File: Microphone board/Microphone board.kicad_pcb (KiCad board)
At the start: 4 copper layers, 155 parts, among them J1 TF-01A, J2 OV2640, J3 NHD-2.4-240320AF-CSXP, J4 TYPE-C 16PIN 2MD(073), M1 MSM261DDB019, M10 MSM261DDB019, M11 MSM261DDB019, M12 MSM261DDB019, M13 MSM261DDB019, M14 MSM261DDB019, M15 MSM261DDB019, M16 MSM261DDB019, M2 MSM261DDB019, M3 MSM261DDB019, M4 MSM261DDB019, M5 MSM261DDB019, M6 MSM261DDB019, M7 MSM261DDB019, M8 MSM261DDB019, M9 MSM261DDB019, Q1 AO3401A, Q2 MMBT3904, U1 STM32H747XIH6, U2 24LC256, U3 TLV320ADC5140IRTWT, U4 TLV320ADC5140IRTWT, U5 TPD6F003, U6 USBLC6-2SC6, U7 AP63203WU, U8 TPS7A2033PDBV, U9 TPS2116DRL, Y1 SX2M25.000M20F30TNN

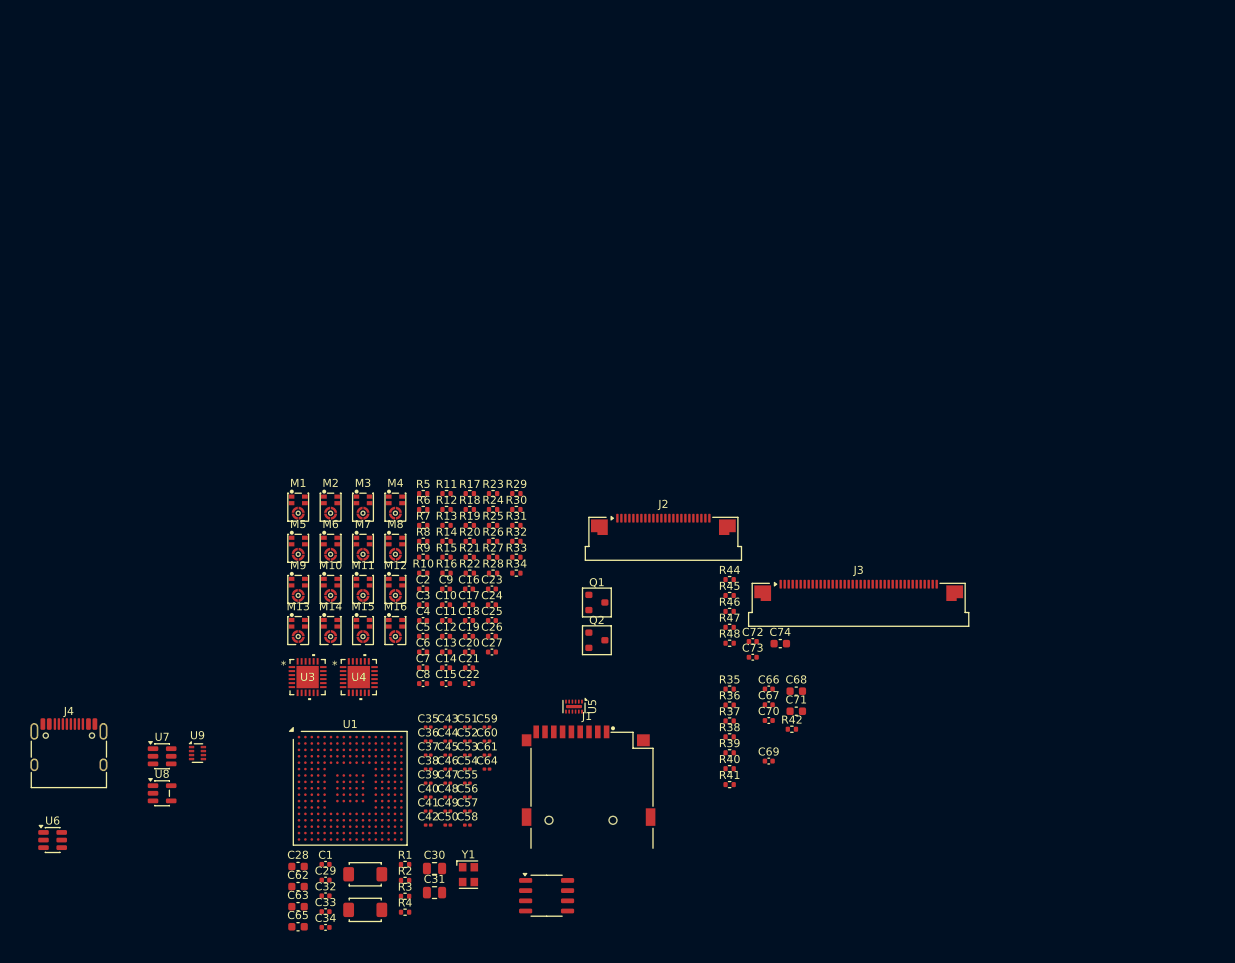
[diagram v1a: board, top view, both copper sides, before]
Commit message: PCB routed
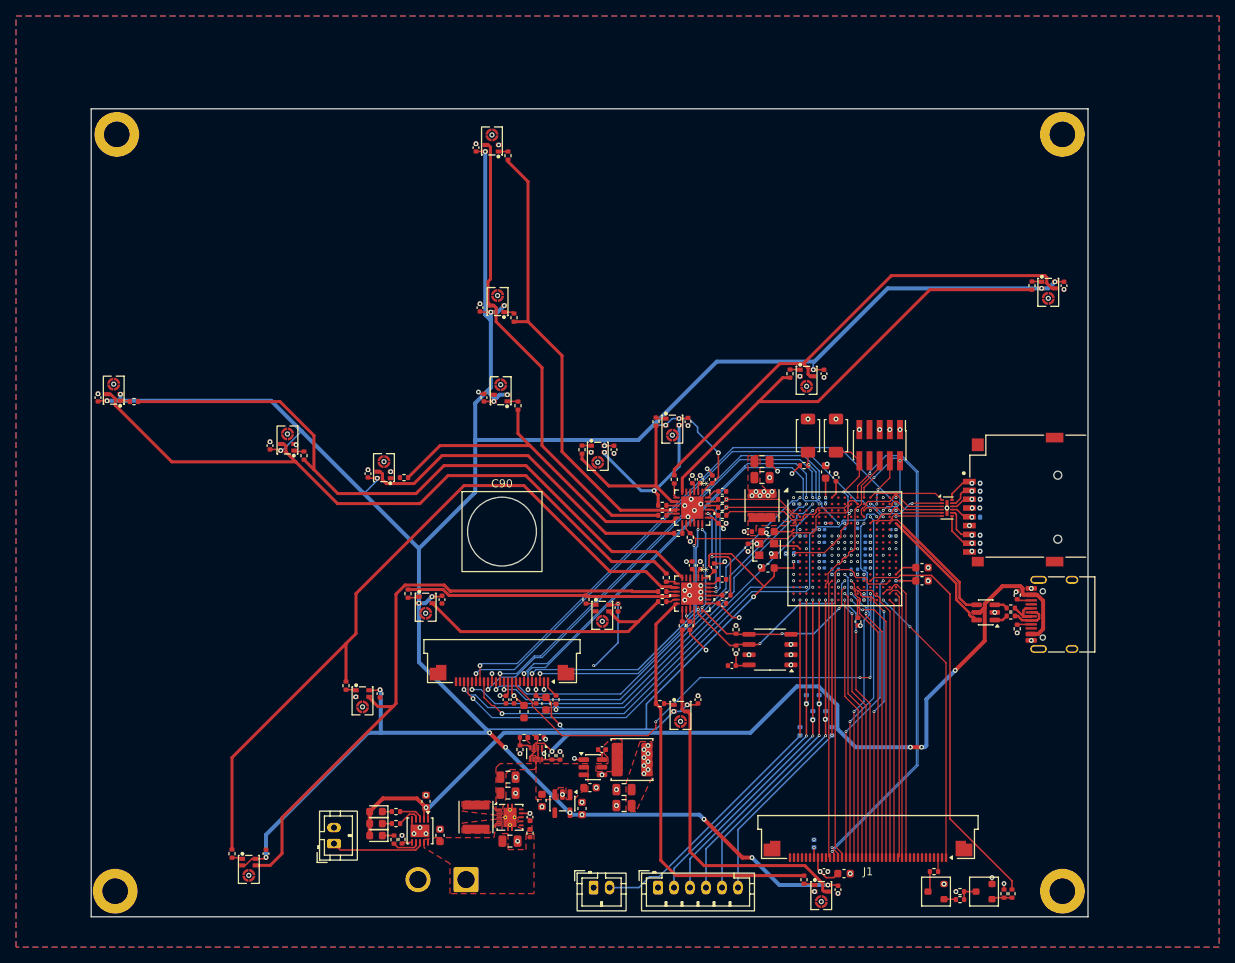
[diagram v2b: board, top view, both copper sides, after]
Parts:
- added BT1: 3.7V 18650, Connector_Wire:SolderWire-1.5sqmm_1x02_P6mm_D1.7mm_OD3mm, F.Cu at (106.2, 135.8)
- added C75: 10u 6.3V, Capacitor_SMD:C_0805_2012Metric, F.Cu at (111.7, 130.9)
- added C76: 100n, Capacitor_SMD:C_0402_1005Metric, F.Cu at (114.2, 127.9)
- added C77: 2.2u, Capacitor_SMD:C_0402_1005Metric, F.Cu at (115.5, 118.0)
- added C78: 10u 6.3V, Capacitor_SMD:C_0805_2012Metric, F.Cu at (111.5, 122.9)
- added C79: 10u 6.3V, Capacitor_SMD:C_0805_2012Metric, F.Cu at (111.5, 124.9)
- added C80: 10u, Capacitor_SMD:C_0603_1608Metric, F.Cu at (121.8, 124.2)
- added C81: 100n, Capacitor_SMD:C_0402_1005Metric, F.Cu at (123.2, 119.5)
- added C82: 22u, Capacitor_SMD:C_0805_2012Metric, F.Cu at (126.0, 124.5)
- added C83: 22u, Capacitor_SMD:C_0805_2012Metric, F.Cu at (126.0, 126.5)
- added C84: 2.2u, Capacitor_SMD:C_0603_1608Metric, F.Cu at (115.8, 125.9)
- added C85: 2.2u, Capacitor_SMD:C_0603_1608Metric, F.Cu at (120.8, 126.9)
- added C86: 1u, Capacitor_SMD:C_0603_1608Metric, F.Cu at (101.2, 126.0)
- added C87: 1u, Capacitor_SMD:C_0603_1608Metric, F.Cu at (103.0, 130.2)
- added C88: 100n, Capacitor_SMD:C_0402_1005Metric, B.Cu at (170.0, 89.3)
- added C89: 100n, Capacitor_SMD:C_0201_0603Metric, B.Cu at (160.3, 98.4)
- added C90: OV2640, Mic_Parts:OV2640, F.Cu at (110.8, 92.2)
- added D1: Green, PCM_JLCPCB:D_0603, F.Cu at (95.0, 130.2)
- added D2: Yellow, PCM_JLCPCB:D_0603, F.Cu at (95.0, 128.8)
- added D3: Red, PCM_JLCPCB:D_0603, F.Cu at (95.0, 127.2)
- added H1: M3 mounting hole, MountingHole:MountingHole_3.2mm_M3_DIN965_Pad, F.Cu at (62.6, 42.6)
- added H2: M3 mounting hole, MountingHole:MountingHole_3.2mm_M3_DIN965_Pad, F.Cu at (62.4, 137.2)
- added H3: M3 mounting hole, MountingHole:MountingHole_3.2mm_M3_DIN965_Pad, F.Cu at (180.8, 137.2)
- added H4: M3 mounting hole, MountingHole:MountingHole_3.2mm_M3_DIN965_Pad, F.Cu at (180.8, 42.6)
- added J5: Trigger, Connector_JST:JST_PH_B2B-PH-K_1x02_P2.00mm_Vertical, F.Cu at (122.2, 136.8)
- added J6: Menu, Connector_JST:JST_PH_B6B-PH-K_1x06_P2.00mm_Vertical, F.Cu at (130.2, 136.8)
- added J7: Conn_ARM_JTAG_SWD_10, Connector_PinHeader_1.27mm:PinHeader_2x05_P1.27mm_Vertical_SMD, F.Cu at (158.0, 81.5)
- added L1: GNR4018S2R2MT, Inductor_SMD:L_Abracon_ASPI-4030S, F.Cu at (143.2, 89.0)
- added L2: GNR4018S2R2MT, Inductor_SMD:L_Abracon_ASPI-4030S, F.Cu at (107.5, 127.9)
- added L3: FNR5040S4R7MT, Inductor_SMD:L_Changjiang_FNR5040S, F.Cu at (127.0, 120.8)
- added R43: 10k, Resistor_SMD:R_0402_1005Metric, B.Cu at (170.0, 90.5)
- added R49: 100k, Resistor_SMD:R_0402_1005Metric, F.Cu at (113.0, 119.5)
- added R50: 100R, Resistor_SMD:R_0402_1005Metric, F.Cu at (114.2, 129.9)
- added R51: 10k, Resistor_SMD:R_0402_1005Metric, F.Cu at (117.0, 120.2)
- added R52: 15k, Resistor_SMD:R_0402_1005Metric, F.Cu at (118.0, 120.2)
- added R53: 470R, Resistor_SMD:R_0402_1005Metric, F.Cu at (97.5, 127.2)
- added R54: 470R, Resistor_SMD:R_0402_1005Metric, F.Cu at (97.5, 128.8)
- added R55: 470R, Resistor_SMD:R_0402_1005Metric, F.Cu at (97.2, 130.8)
- added R56: 5k1, Resistor_SMD:R_0402_1005Metric, F.Cu at (175.2, 104.4)
- added R57: 5k1, Resistor_SMD:R_0402_1005Metric, F.Cu at (175.2, 100.2)
- added R58: 22R, Resistor_SMD:R_0402_1005Metric, F.Cu at (174.3, 102.8)
- added R59: 22R, Resistor_SMD:R_0402_1005Metric, F.Cu at (174.3, 101.8)
- added R60: 1k, Resistor_SMD:R_0402_1005Metric, F.Cu at (98.2, 130.7)
- added R61: 10k, Resistor_SMD:R_0402_1005Metric, B.Cu at (148.0, 117.2)
- added R62: 10k, Resistor_SMD:R_0402_1005Metric, B.Cu at (152.0, 117.2)
- added R63: 10k, Resistor_SMD:R_0402_1005Metric, B.Cu at (151.2, 115.2)
- added R64: 10k, Resistor_SMD:R_0402_1005Metric, B.Cu at (150.4, 113.2)
- added R65: 10k, Resistor_SMD:R_0402_1005Metric, B.Cu at (149.6, 115.2)
- added R66: 10k, Resistor_SMD:R_0402_1005Metric, B.Cu at (148.8, 113.2)
- added TH1: 10k, Connector_JST:JST_PH_B2B-PH-K_1x02_P2.00mm_Vertical, F.Cu at (89.8, 131.2)
- added U10: TPS7A2033PDBV, Package_TO_SOT_SMD:SOT-23-5, F.Cu at (118.3, 126.2)
- added U11: USBLC6-2SC6, Package_TO_SOT_SMD:SOT-23-6, F.Cu at (171.2, 102.3)
- C1: value 100n -> 220pF
- C10, C11, C12, C13, C14, C16, C17, C18, C19, C20, C21, C22, C23, C24, C25, C26, C27, C8, C9: footprint Capacitor_SMD:C_0402_1005Metric -> Capacitor_SMD:C_0201_0603Metric; moved to B.Cu
- C15: value 100n -> 1u; footprint Capacitor_SMD:C_0402_1005Metric -> Capacitor_SMD:C_0603_1608Metric
- C2: footprint Capacitor_SMD:C_0402_1005Metric -> Capacitor_SMD:C_0603_1608Metric
- C28: value 4.7u -> 100n; footprint Capacitor_SMD:C_0603_1608Metric -> Capacitor_SMD:C_0201_0603Metric; moved to B.Cu
- C29: value 220pF -> 100n; footprint Capacitor_SMD:C_0402_1005Metric -> Capacitor_SMD:C_0201_0603Metric; moved to B.Cu
- C30, C31: value 10u -> 100n; footprint Capacitor_SMD:C_0805_2012Metric -> Capacitor_SMD:C_0201_0603Metric; moved to B.Cu
- C32, C33, C34: value 2.2u -> 100n; footprint Capacitor_SMD:C_0402_1005Metric -> Capacitor_SMD:C_0201_0603Metric; moved to B.Cu
- C35, C36, R1, R41, R42: moved to B.Cu
- C37: value 100n -> 4.7u; footprint Capacitor_SMD:C_0201_0603Metric -> Capacitor_SMD:C_0603_1608Metric
- C38: value 100n -> 1u; footprint Capacitor_SMD:C_0201_0603Metric -> Capacitor_SMD:C_0603_1608Metric
- C39, C40, C41, C42, C43, C44, C45, C46, C47, C48, C49, C50, C51, C52, C53, C54, C55, C56, C59, C60, C64: footprint Capacitor_SMD:C_0201_0603Metric -> Capacitor_SMD:C_0402_1005Metric
- C4, C69: value 100n -> 4.7u; footprint Capacitor_SMD:C_0402_1005Metric -> Capacitor_SMD:C_0603_1608Metric
- C57, C58, C61: value 100n -> 2.2u; footprint Capacitor_SMD:C_0201_0603Metric -> Capacitor_SMD:C_0402_1005Metric
- C6: value 100n -> 10u; footprint Capacitor_SMD:C_0402_1005Metric -> Capacitor_SMD:C_0805_2012Metric
- C62: value 4.7u -> 2.2u; footprint Capacitor_SMD:C_0603_1608Metric -> Capacitor_SMD:C_0402_1005Metric
- C63, C65: value 1u -> 100n; footprint Capacitor_SMD:C_0603_1608Metric -> Capacitor_SMD:C_0402_1005Metric
- C68: value 4.7u -> 100n; footprint Capacitor_SMD:C_0603_1608Metric -> Capacitor_SMD:C_0402_1005Metric; moved to B.Cu
- C7: value 2.2u -> 10u; footprint Capacitor_SMD:C_0402_1005Metric -> Capacitor_SMD:C_0805_2012Metric
- J1: value TF-01A -> NHD-2.4-240320AF-CSXP; footprint Mic_Parts:TF-01A -> Connector_FFC-FPC:Amphenol_F32R-1A7x1-11040_1x40-1MP_P0.5mm_Horizontal
- J2: footprint Connector_FFC-FPC:Amphenol_F32R-1A7x1-11024_1x24-1MP_P0.5mm_Horizontal -> Connector_FFC-FPC:Amphenol_F32Q-1A7x1-11024_1x24-1MP_P0.5mm_Horizontal
- J3: value NHD-2.4-240320AF-CSXP -> TF-01A; footprint Connector_FFC-FPC:Amphenol_F32R-1A7x1-11040_1x40-1MP_P0.5mm_Horizontal -> Mic_Parts:TF-01A
- Q1: value AO3401A -> MMBT3904
- Q2: value MMBT3904 -> AO3401A
- R10, R11, R12, R13, R14, R15, R16, R17, R18, R19, R20, R21, R22, R23, R24, R29, R30, R31, R32, R7, R8, R9: value 33R -> 22R
- R2: value 10k -> 2k2
- R33, R34: value 33R -> 10k
- R35: value 10k -> 1k
- R37: value 10k -> 4k7
- R38: value 10k -> 10R
- R39: value 10k -> 2R
- R4: value 2k2 -> 10k
- R44: value 10R -> 10k; moved to B.Cu
- R45: value 4k7 -> 10k; moved to B.Cu
- R46: value 2R -> 10k; moved to B.Cu
- R47: value 1k -> 10k; moved to B.Cu
- R48: value 10k -> 240k
- R5, R6: value 10k -> 22R
- U6: value USBLC6-2SC6 -> TPS63001; footprint Package_TO_SOT_SMD:SOT-23-6 -> Package_SON:Texas_DRC0010J_ThermalVias
- U7: value AP63203WU -> TPS2116DRL; footprint Package_TO_SOT_SMD:TSOT-23-6 -> Package_TO_SOT_SMD:SOT-583-8
- U8: value TPS7A2033PDBV -> AP63203WU; footprint Package_TO_SOT_SMD:SOT-23-5 -> Package_TO_SOT_SMD:TSOT-23-6
- U9: value TPS2116DRL -> MCP73833-xxx-MF; footprint Package_TO_SOT_SMD:SOT-583-8 -> Package_DFN_QFN:DFN-10-1EP_3x3mm_P0.5mm_EP1.58x2.35mm
- moved J4 125.6 mm to (180.9, 102.6), turned to 90 degrees
- moved C49 101.2 mm to (181.0, 61.5), turned to -90 degrees
- moved M1 97.5 mm to (179.0, 63.1)
- moved C32 84.0 mm to (159.7, 92.8), turned to 180 degrees
- moved C28 82.3 mm to (156.5, 92.8), turned to 180 degrees
- moved C34 82.2 mm to (151.2, 88.3), turned to -90 degrees
- moved S2 81.1 mm to (149.0, 80.2), turned to -90 degrees
- moved S1 80.4 mm to (152.5, 80.2), turned to 90 degrees
- moved C29 79.4 mm to (156.5, 94.4), turned to 180 degrees
- moved R13 79.1 mm to (177.0, 61.5), turned to -90 degrees
- moved C33 77.3 mm to (150.7, 93.6)
- moved C65 76.2 mm to (137.0, 85.7), turned to 90 degrees
- moved R4 74.9 mm to (148.5, 84.0), turned to 180 degrees
- moved C41 73.7 mm to (151.0, 72.5), turned to -90 degrees
- moved C31 73.1 mm to (159.7, 92.0), turned to 180 degrees
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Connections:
- net Net-(J4-D+-PadA6) renamed /USB/USB_IN_P
- net Net-(J4-D--PadA7) renamed /USB/USB_IN_N
- C1 pad 1: +3V3 -> Net-(U1A-VLXSMPS)
- C10 pad 1: +3V3A -> +3V3
- C12 pad 1: +3V3A -> +3V3
- C13 pad 1: +3V3A -> +3V3
- C14 pad 1: +3V3A -> +3V3
- C16 pad 1: +3V3A -> +3V3
- C17 pad 1: +3V3A -> +3V3
- C18 pad 1: +3V3A -> +3V3
- C19 pad 1: +3V3A -> +3V3
- C2 pad 1: Net-(U3B-AREG) -> Net-(U1A-VCAPDSI)
- C20 pad 1: +3V3A -> +3V3
- C21 pad 1: +3V3A -> +3V3
- C22 pad 1: +3V3A -> +3V3
- C23 pad 1: +3V3A -> +3V3
- C24 pad 1: +3V3A -> +3V3
- C27 pad 1: +3V3A -> +3V3
- C28 pad 1: Net-(U1A-VDDSMPS) -> +3V3
- C29 pad 1: Net-(U1A-VLXSMPS) -> +3V3
- C3 pad 1: Net-(U4B-AREG) -> Net-(C3-Pad1)
- C32 pad 1: Net-(C32-Pad1) -> +3V3
- C33 pad 1: Net-(C32-Pad1) -> +3V3
- C34 pad 1: Net-(U1A-VCAPDSI) -> +3V3
- C4 pad 1: Net-(U3B-VREF) -> Net-(U1A-VDDSMPS)
- C41 pad 1: +3V3 -> +3V3A
- C42 pad 1: +3V3 -> +3V3A
- C43 pad 1: +3V3 -> +3V3A
- C44 pad 1: +3V3 -> +3V3A
- C45 pad 1: +3V3 -> +3V3A
- C46 pad 1: +3V3 -> +3V3A
- C47 pad 1: +3V3 -> +3V3A
- C48 pad 1: +3V3 -> +3V3A
- C49 pad 1: +3V3 -> +3V3A
- C5 pad 1: Net-(U3B-DREG) -> Net-(C3-Pad1)
- C50 pad 1: +3V3 -> +3V3A
- C51 pad 1: +3V3 -> +3V3A
- C52 pad 1: +3V3 -> +3V3A
- C53 pad 1: +3V3 -> +3V3A
- C54 pad 1: +3V3 -> +3V3A
- C55 pad 1: +3V3 -> +3V3A
- C56 pad 1: +3V3 -> +3V3A
- C57 pad 1: +3V3 -> Net-(U3B-AREG)
- C58 pad 1: +3V3 -> Net-(U4B-AREG)
- C59 pad 1: +3V3 -> Net-(U3B-VREF)
- C6 pad 1: Net-(U4B-VREF) -> +3V3
- C60 pad 1: +3V3 -> Net-(U4B-VREF)
- C61 pad 1: +3V3 -> Net-(U3B-DREG)
- C62 pad 1: +3V3 -> Net-(U4B-DREG)
- C64 pad 1: +3V3A -> +3V3
- C66 pad 1: +3V3 -> +3V3A
- C7 pad 1: Net-(U4B-DREG) -> +3V3
- C8 pad 1: +3V3A -> +3V3
- C9 pad 1: +3V3A -> +3V3
- J1 pad 1: Net-(J1-DAT2) -> /MCU/TEAR
- J1 pad 2: Net-(J1-DAT3/CD) -> GND
- J1 pad 3: Net-(J1-CMD) -> /Display/LIGHT
- J1 pad 4: +3V3 -> GND
- J1 pad 5: Net-(J1-CLK) -> GND
- J1 pad 7: Net-(J1-DAT0) -> GND
- J1 pad 8: Net-(J1-DAT1) -> GND
- J1 pad 9: /MCU/SD_DET -> GND
- J2 pad 18: /MCU/DCMI_D7 -> /MCU/DCMI_D4
- J3 pad 1: GND -> /SD/SD_D2F
- J3 pad 2: unconnected-(J3-Pin_2-Pad2) -> /SD/SD_D3F
- J3 pad 3: unconnected-(J3-Pin_3-Pad3) -> /SD/SD_CMDF
- J3 pad 4: unconnected-(J3-Pin_4-Pad4) -> +3V3
- J3 pad 5: unconnected-(J3-Pin_5-Pad5) -> /SD/SD_CLKF
- J3 pad 6: unconnected-(J3-Pin_6-Pad6) -> GND
- J3 pad 7: +3V3 -> /SD/SD_D0F
- J3 pad 8: +3V3 -> /SD/SD_D1F
- J3 pad 9: GND -> /MCU/SD_DET
- M10 pad 4: /Microphones/CH6_CLK -> /Microphones/CH5_CLK
- M11 pad 2: GND -> +3V3A
- M11 pad 4: /Microphones/CH7_CLK -> /Microphones/CH6_CLK
- M12 pad 4: /Microphones/CH8_CLK -> /Microphones/CH6_CLK
- M13 pad 4: unconnected-(M13-CLK-Pad4) -> /Microphones/CH7_CLK
- M14 pad 2: +3V3A -> GND
- M14 pad 4: /Microphones/CH5_CLK -> /Microphones/CH7_CLK
- M15 pad 4: /Microphones/CH6_CLK -> /Microphones/CH8_CLK
- M16 pad 2: +3V3A -> GND
- M3 pad 2: GND -> +3V3A
- M4 pad 2: +3V3A -> GND
- M5 pad 2: GND -> +3V3A
- M6 pad 4: /Microphones/CH4_CLK -> /Microphones/CH3_CLK
- M7 pad 4: /Microphones/CH3_CLK -> /Microphones/CH4_CLK
- M8 pad 2: +3V3A -> GND
- M9 pad 2: GND -> +3V3A
- Q1 pad 1: Net-(Q1-G) -> Net-(Q1-B)
- Q1 pad 2: +3V3 -> GND
- Q1 pad 3: Net-(Q1-D) -> Net-(Q1-C)
- Q2 pad 1: Net-(Q2-B) -> Net-(Q2-G)
- Q2 pad 2: GND -> +3V3
- Q2 pad 3: Net-(Q2-C) -> Net-(Q2-D)
- R1 pad 1: /MCU/BOOT0 -> +3V3
- R1 pad 2: GND -> /MCU/NRST
- R10 pad 1: /Microphones/CH4_CLK -> Net-(M12-DAT)
- R10 pad 2: Net-(U3A-IN4M_GPO4) -> /Microphones/CH6_DAT
- R11 pad 1: /Microphones/CH5_CLK -> Net-(M14-DAT)
- R11 pad 2: Net-(U4A-IN1M_GPO1) -> /Microphones/CH7_DAT
- R12 pad 1: /Microphones/CH6_CLK -> Net-(M16-DAT)
- R12 pad 2: Net-(U4A-IN2M_GPO2) -> /Microphones/CH8_DAT
- R13 pad 1: /Microphones/CH7_CLK -> Net-(M1-DAT)
- R13 pad 2: Net-(U4A-IN3M_GPO3) -> /Microphones/CH1_DAT
- R14 pad 1: /Microphones/CH8_CLK -> Net-(M3-DAT)
- R14 pad 2: Net-(U4A-IN4M_GPO4) -> /Microphones/CH2_DAT
- R15 pad 1: Net-(M1-DAT) -> Net-(M5-DAT)
- R15 pad 2: /Microphones/CH1_DAT -> /Microphones/CH3_DAT
- R16 pad 1: Net-(M2-DAT) -> Net-(M7-DAT)
- R16 pad 2: /Microphones/CH1_DAT -> /Microphones/CH4_DAT
- R17 pad 1: Net-(M4-DAT) -> Net-(M9-DAT)
- R17 pad 2: /Microphones/CH2_DAT -> /Microphones/CH5_DAT
- R18 pad 1: Net-(M3-DAT) -> Net-(M11-DAT)
- R18 pad 2: /Microphones/CH2_DAT -> /Microphones/CH6_DAT
- R19 pad 1: Net-(M7-DAT) -> Net-(M13-DAT)
- R19 pad 2: /Microphones/CH3_DAT -> /Microphones/CH7_DAT
- R2 pad 2: /MCU/NRST -> /MCU/I2C4_SDA
- R20 pad 1: Net-(M5-DAT) -> Net-(M15-DAT)
- R20 pad 2: /Microphones/CH3_DAT -> /Microphones/CH8_DAT
- R21 pad 1: Net-(M8-DAT) -> /Microphones/CH5_CLK
- R21 pad 2: /Microphones/CH4_DAT -> Net-(U4A-IN1M_GPO1)
- R22 pad 1: Net-(M6-DAT) -> /Microphones/CH6_CLK
- R22 pad 2: unconnected-(R22-Pad2) -> Net-(U4A-IN2M_GPO2)
- R23 pad 1: Net-(M13-DAT) -> /Microphones/CH7_CLK
- R23 pad 2: /Microphones/CH4_DAT -> Net-(U4A-IN3M_GPO3)
- R24 pad 1: Net-(M9-DAT) -> /Microphones/CH8_CLK
- R24 pad 2: /Microphones/CH5_DAT -> Net-(U4A-IN4M_GPO4)
- R25 pad 1: Net-(M14-DAT) -> /Microphones/CH1_CLK
- R25 pad 2: /Microphones/CH5_DAT -> Net-(U3A-IN1M_GPO1)
- R26 pad 1: Net-(M10-DAT) -> /Microphones/CH2_CLK
- R26 pad 2: /Microphones/CH6_DAT -> Net-(U3A-IN2M_GPO2)
- R27 pad 1: Net-(M15-DAT) -> /Microphones/CH3_CLK
- R27 pad 2: /Microphones/CH6_DAT -> Net-(U3A-IN3M_GPO3)
- R28 pad 1: Net-(M11-DAT) -> /Microphones/CH4_CLK
- R28 pad 2: /Microphones/CH7_DAT -> Net-(U3A-IN4M_GPO4)
- R29 pad 1: Net-(M16-DAT) -> Net-(U4A-SDOUT)
- R29 pad 2: /Microphones/CH8_DAT -> Net-(U3A-GPIO1)
- R3 pad 2: /MCU/I2C4_SDA -> /MCU/I2C4_SCL
- R30 pad 1: Net-(M12-DAT) -> Net-(U3A-SDOUT)
- R30 pad 2: /Microphones/CH8_DAT -> /MCU/SAI_SD
- R31 pad 1: Net-(U3A-SDOUT) -> Net-(U3A-FSYNC)
- R31 pad 2: /MCU/SAI_SD -> /MCU/SAI_FS
- R32 pad 1: Net-(U3A-FSYNC) -> Net-(U3A-BCLK)
- R32 pad 2: /MCU/SAI_FS -> /MCU/SAI_SCK
- R33 pad 1: Net-(U3A-BCLK) -> +3V3
- R33 pad 2: /MCU/SAI_SCK -> /MCU/SHDNZ
- R34 pad 1: Net-(U4A-SDOUT) -> +3V3
- R34 pad 2: Net-(U3A-GPIO1) -> /MCU/SHDNZ
- R35 pad 1: +3V3 -> /MCU/LIGHT_PWM
- R35 pad 2: /MCU/SD_DET -> Net-(Q1-B)
- R36 pad 1: +3V3 -> GND
- R36 pad 2: Net-(J1-DAT2) -> Net-(Q1-B)
- R37 pad 1: +3V3 -> Net-(Q1-C)
- R37 pad 2: Net-(J1-DAT3/CD) -> +3V3
- R38 pad 1: +3V3 -> Net-(Q1-C)
- R38 pad 2: Net-(J1-CMD) -> Net-(Q2-G)
- R39 pad 1: +3V3 -> Net-(Q2-D)
- R39 pad 2: Net-(J1-CLK) -> /Display/LIGHT
- R4 pad 1: +3V3 -> /MCU/BOOT0
- R4 pad 2: /MCU/I2C4_SCL -> GND
- R40 pad 1: +3V3 -> GND
- R40 pad 2: Net-(J1-DAT0) -> Net-(J2-Pin_1)
- R41 pad 2: Net-(J1-DAT1) -> /SD/SD_D1F
- R42 pad 1: GND -> +3V3
- R42 pad 2: Net-(J2-Pin_1) -> /SD/SD_D0F
- R44 pad 1: Net-(Q2-C) -> +3V3
- R44 pad 2: Net-(Q1-G) -> /SD/SD_CMDF
- R45 pad 1: Net-(Q2-C) -> +3V3
- R45 pad 2: +3V3 -> /SD/SD_D3F
- R46 pad 1: Net-(Q1-D) -> +3V3
- R46 pad 2: /Display/LIGHT -> /MCU/SD_DET
- R47 pad 1: /MCU/LIGHT_PWM -> +3V3
- R47 pad 2: Net-(Q2-B) -> /SD/SD_D2F
- R48 pad 1: GND -> VBUS
- R48 pad 2: Net-(Q2-B) -> Net-(U7-PR1)
- R5 pad 1: +3V3 -> Net-(M2-DAT)
- R5 pad 2: /Microphones/SHDNZ -> /Microphones/CH1_DAT
- R6 pad 1: +3V3 -> Net-(M4-DAT)
- R6 pad 2: /Microphones/SHDNZ -> /Microphones/CH2_DAT
- R7 pad 1: /Microphones/CH1_CLK -> Net-(M6-DAT)
- R7 pad 2: Net-(U3A-IN1M_GPO1) -> /Microphones/CH3_DAT
- R8 pad 1: /Microphones/CH2_CLK -> Net-(M8-DAT)
- R8 pad 2: Net-(U3A-IN2M_GPO2) -> /Microphones/CH4_DAT
- R9 pad 1: /Microphones/CH3_CLK -> Net-(M10-DAT)
- R9 pad 2: Net-(U3A-IN3M_GPO3) -> /Microphones/CH5_DAT
- S1 pad 1: +3V3 -> /MCU/NRST
- S1 pad 2: /MCU/BOOT0 -> GND
- S2 pad 1: /MCU/NRST -> +3V3
- S2 pad 2: GND -> /MCU/BOOT0
- U1 pad A10: /MCU/DCMI_VSYNC -> unconnected-(U1D-PG9-PadA10)
- U1 pad A3: unconnected-(U1E-PI5-PadA3) -> /MCU/DCMI_VSYNC
- U1 pad A7: Net-(C32-Pad1) -> Net-(C3-Pad1)
- U1 pad B10: unconnected-(U1E-PJ15-PadB10) -> /MCU/SHDNZ
- U1 pad B14: unconnected-(U1B-SWCLK-PadB14) -> /MCU/SWCLK
- U1 pad C15: unconnected-(U1B-SWDIO-PadC15) -> /MCU/SWDIO
- U1 pad D17: Net-(C32-Pad1) -> Net-(C3-Pad1)
- U1 pad E16: /MCU/USB_DP -> /MCU/USB_P
- U1 pad E17: /MCU/USB_DM -> /MCU/USB_N
- U1 pad E7: unconnected-(U1A-PDR_ON-PadE7) -> +3V3
- U1 pad R11: unconnected-(U1D-PE15-PadR11) -> /MCU/FMC_D12
- U1 pad R6: unconnected-(U1C-PB2-PadR6) -> /MCU/SWO
- U1 pad U10: unconnected-(U1D-PE14-PadU10) -> /MCU/FMC_D11
- U1 pad U11: Net-(C32-Pad1) -> Net-(C3-Pad1)
- U1 pad U2: unconnected-(U1C-PA3-PadU2) -> /MCU/TRIGGER
- U1 pad U3: unconnected-(U1C-PA4-PadU3) -> /MCU/LEFT
- U1 pad U4: unconnected-(U1C-PC5-PadU4) -> /MCU/DOWN
- U1 pad U5: unconnected-(U1C-PB0-PadU5) -> /MCU/BUTTON
- U1 pad U6: unconnected-(U1E-PJ3-PadU6) -> /MCU/RIGHT
- U1 pad U7: unconnected-(U1E-PJ4-PadU7) -> /MCU/UP
- U3 pad 14: /Microphones/SHDNZ -> /MCU/SHDNZ
- U4 pad 14: /Microphones/SHDNZ -> /MCU/SHDNZ
- U5 pad 1: /MCU/SD_D0 -> /MCU/SD_D2
- U5 pad 10: Net-(J1-CMD) -> /SD/SD_CMDF
- U5 pad 11: Net-(J1-DAT3/CD) -> /SD/SD_D3F
- U5 pad 12: Net-(J1-DAT2) -> /SD/SD_D2F
- U5 pad 7: Net-(J1-DAT1) -> /SD/SD_D1F
- U5 pad 8: Net-(J1-DAT0) -> /SD/SD_D0F
- U5 pad 9: Net-(J1-CLK) -> /SD/SD_CLKF
- U6 pad 1: Net-(R50-Pad2) -> +5VB
- U6 pad 2: GND -> Net-(U6-L2)
- U6 pad 3: Net-(R51-Pad2) -> GND
- U6 pad 4: /MCU/USB_DP -> Net-(U6-L1)
- U6 pad 5: VBUS -> VBAT
- U6 pad 6: /MCU/USB_DM -> Net-(U6-EN)
- U7 pad 1: +3V3 -> GND
- U7 pad 3: +5V -> VBUS
- U7 pad 4: GND -> Net-(U7-PR1)
- U7 pad 5: Net-(U7-SW) -> VBUS
- U7 pad 6: Net-(U7-BST) -> +5VB
- U8 pad 1: +5V -> +3V3
- U8 pad 2: GND -> +5V
- U8 pad 4: unconnected-(U8-NC-Pad4) -> GND
- U8 pad 5: +3V3A -> Net-(U8-SW)
- U9 pad 1: GND -> VBUS
- U9 pad 2: +5V -> VBUS
- U9 pad 3: VBUS -> Net-(U9-STAT1)
- U9 pad 5: VBUS -> GND
- U9 pad 6: unconnected-(U9-VIN2-Pad6) -> Net-(U9-PROG)
- U9 pad 7: +5V -> Net-(U9-~{PG})
- U9 pad 8: /MCU/PWR_STATUS -> Net-(U9-THERM)
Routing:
- net +3V3A: track 0.00 -> 453.1 mm, vias 0 -> 35
- net VBUS: track 0.00 -> 133.0 mm, vias 0 -> 5
- net /Microphones/CH6_DAT: track 0.00 -> 94.1 mm
- net /Microphones/CH5_CLK: track 0.00 -> 85.8 mm
- net /Microphones/CH5_DAT: track 0.00 -> 84.3 mm
- net /Microphones/CH6_CLK: track 0.00 -> 79.4 mm
- net /MCU/DCMI_D1: track 0.00 -> 68.8 mm, vias 0 -> 2
- net /MCU/DCMI_D4: track 0.00 -> 68.2 mm, vias 0 -> 2
- net /MCU/DCMI_D0: track 0.00 -> 66.8 mm, vias 0 -> 2
- net /MCU/FMC_NWE: track 0.00 -> 64.3 mm, vias 0 -> 2
- net /MCU/FMC_NOE: track 0.00 -> 63.0 mm, vias 0 -> 2
- net /Microphones/CH1_CLK: track 0.00 -> 61.8 mm
- net /MCU/DCMI_HSYNC: track 0.00 -> 61.6 mm, vias 0 -> 4
- net /MCU/I2C4_SCL: track 0.00 -> 60.6 mm, vias 0 -> 5
- net /Microphones/CH1_DAT: track 0.00 -> 60.3 mm
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- added copper zone on F.Cu, net +3V3
- added copper zone on In1.Cu, net +3V3
- added copper zone on F.Cu, net +5V
- added copper zone on F.Cu, net +5VB
- added copper zone on B.Cu, net GND
- added copper zone on F.Cu, net GND
- added copper zone on In2.Cu, net GND
- added copper zone on F.Cu, net Net-(U1A-VLXSMPS)
- added copper zone on F.Cu, net Net-(U6-EN)
- added copper zone on F.Cu, net Net-(U6-L1)
- added copper zone on F.Cu, net Net-(U6-L2)
- added copper zone on F.Cu, net Net-(U8-SW)
- added copper zone on F.Cu, net VBAT
- added copper zone on F.Cu, net VBUS
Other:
- board outline added: 124.6 x 101 mm
